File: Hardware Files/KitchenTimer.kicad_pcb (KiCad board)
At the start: 2 copper layers, 100 x 100 mm, 89 parts, among them J1 Conn_01x04, J2 USB_B_Micro, J3 Battery, Q1 P 1V 250uA 4A SOT-23, Q10 Q_NMOS_GSD, Q11 Q_NMOS_GSD, Q12 Q_NMOS_GSD, Q13 Q_NMOS_GSD, Q14 -30V 12A 14mΩ @ 8A, Q15 20V 7.5A 24mΩ @ 2.5Vgs, Q2 P 1V 250uA 4A SOT-23, Q3 P 1V 250uA 4A SOT-23, Q4 P 1V 250uA 4A SOT-23, Q5 P 1V 250uA 4A SOT-23, Q6 Q_NMOS_GSD, Q7 Q_NMOS_GSD, Q8 Q_NMOS_GSD, Q9 Q_NMOS_GSD, SW1 SW_SPST, SW2 SW_SPST, SW3 SW_Push_Dual, SW4 SW_Push_Dual, SW5 SW_Push_Dual, SW6 SW_Push_Dual, U1 74HC595, U2 74HC595, U3 ESP-WROOM-02D, U4 AP34063S8G-13, U5 TP4056, U6 AP9101CK6, U7 NCP1117ST50T3G, U8 NCP1117ST33T3G

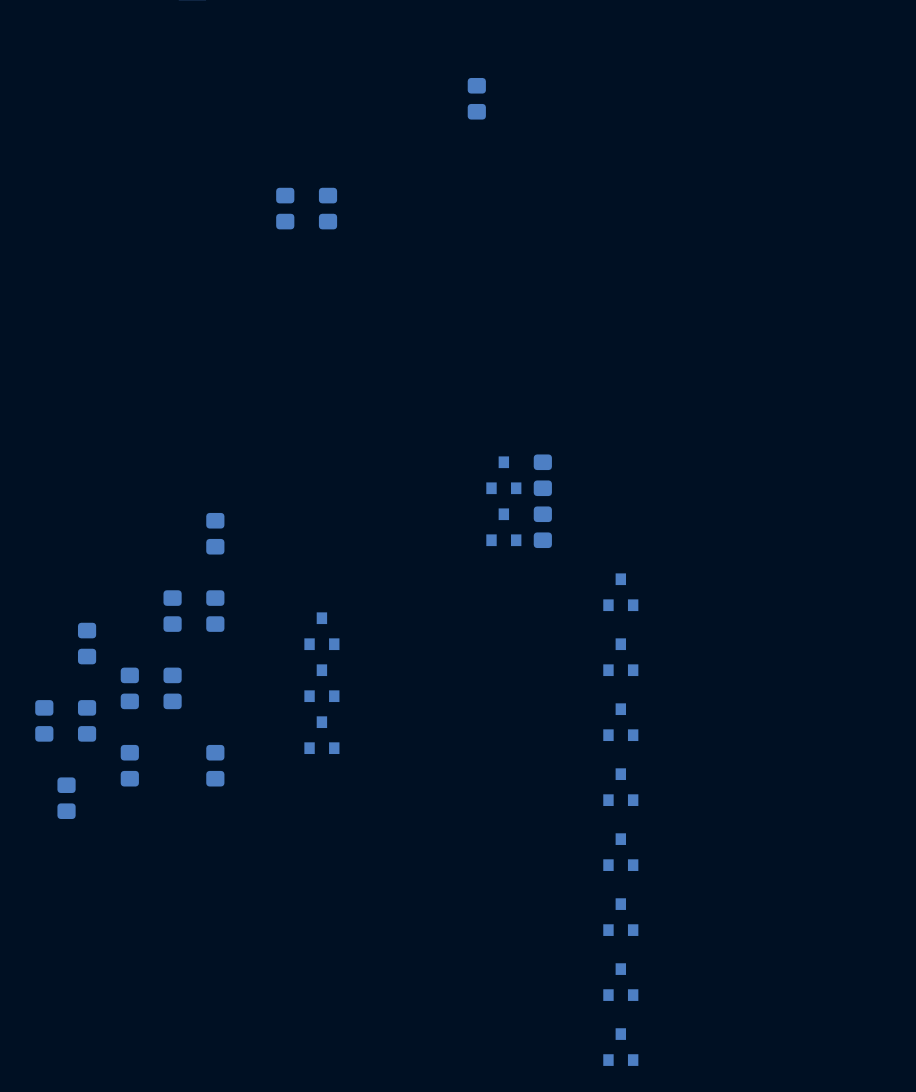
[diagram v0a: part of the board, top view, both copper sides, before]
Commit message: fix ground naming
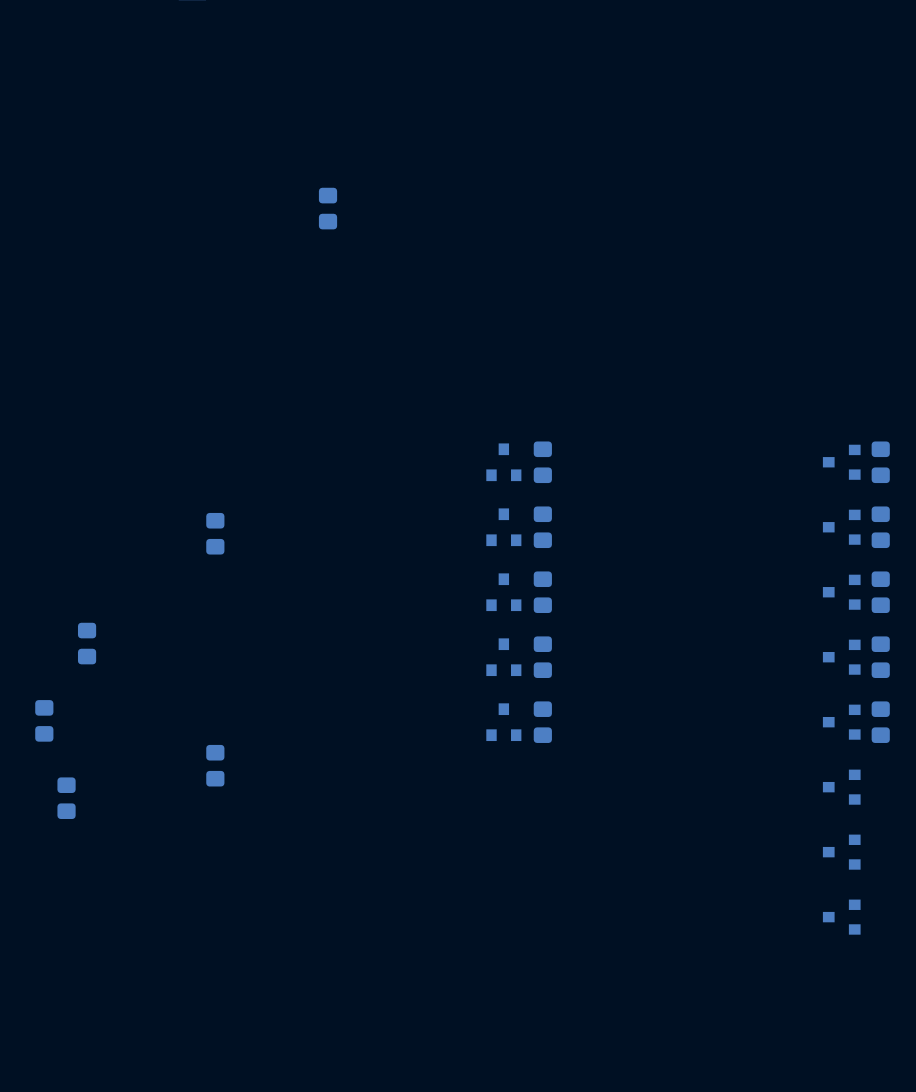
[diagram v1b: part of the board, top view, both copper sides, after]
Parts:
- moved R24 62.9 mm to (218.0, 67.0), turned to 270 degrees
- moved R25 58.3 mm to (218.0, 72.0), turned to 270 degrees
- moved R26 57.4 mm to (218.0, 77.0), turned to 270 degrees
- moved R27 55.2 mm to (218.0, 82.0), turned to 270 degrees
- moved R23 52.5 mm to (218.0, 62.0), turned to 270 degrees
- moved R20 38.3 mm to (192.0, 72.0)
- moved R22 32.0 mm to (192.0, 82.0)
- moved R21 28.6 mm to (192.0, 77.0)
- moved Q10 19.7 mm to (215.0, 82.0), turned to 180 degrees
- moved Q11 19.7 mm to (215.0, 87.0), turned to 180 degrees
- moved Q12 19.7 mm to (215.0, 92.0), turned to 180 degrees
- moved Q13 19.7 mm to (215.0, 97.0), turned to 180 degrees
- moved Q6 19.7 mm to (215.0, 62.0), turned to 180 degrees
- moved Q7 19.7 mm to (215.0, 67.0), turned to 180 degrees
- moved Q8 19.7 mm to (215.0, 72.0), turned to 180 degrees
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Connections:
- net LED_':'_Sink renamed GND

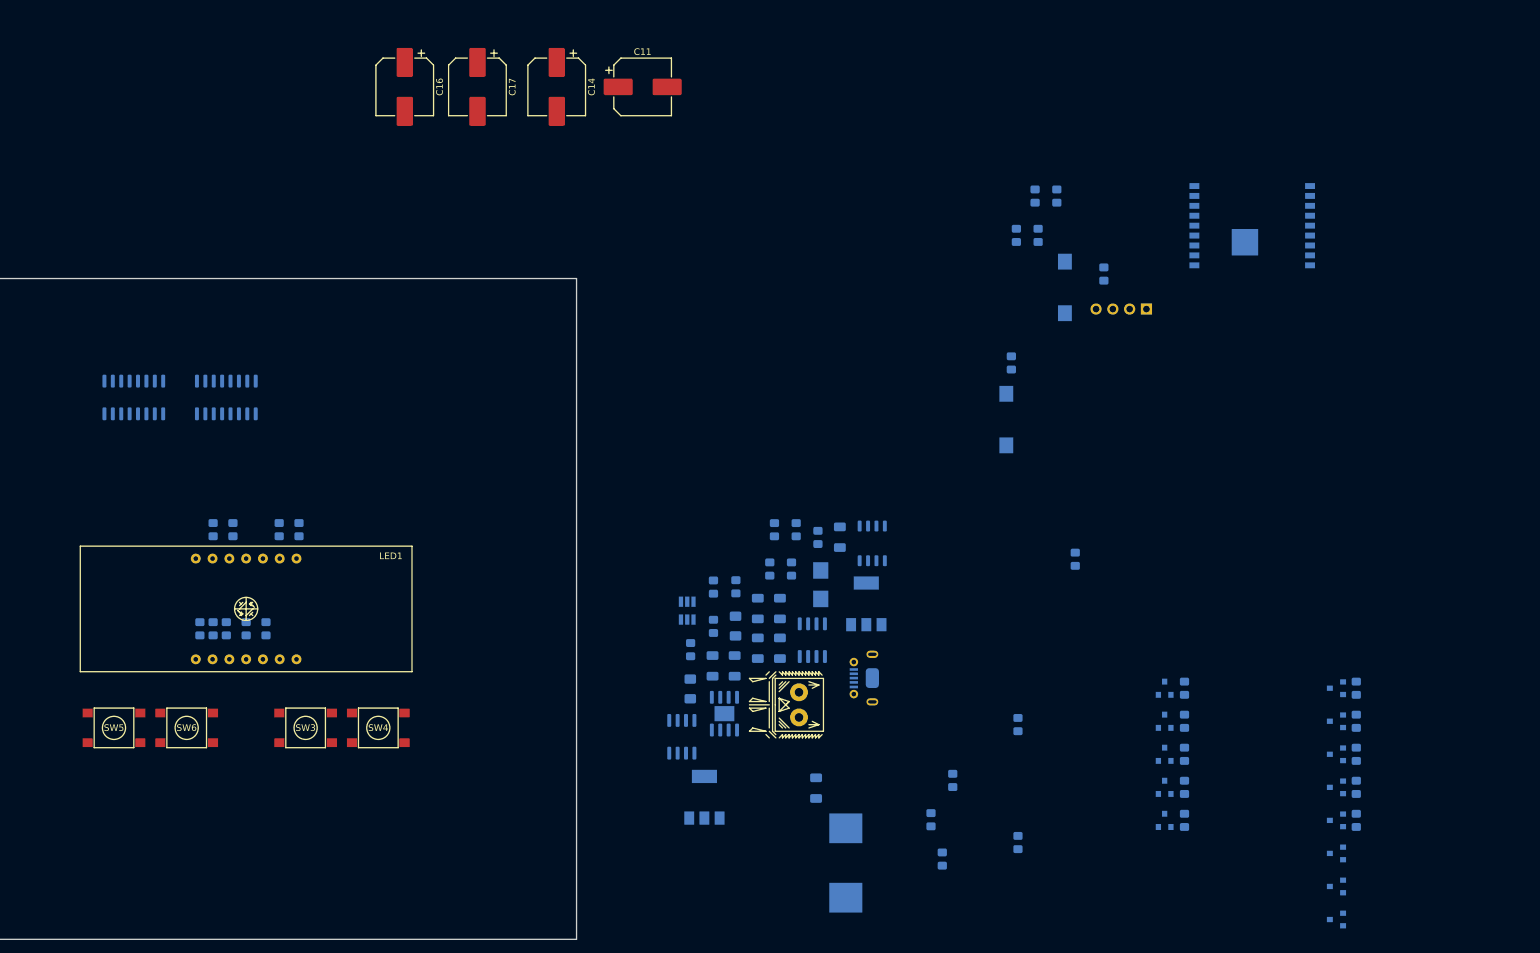
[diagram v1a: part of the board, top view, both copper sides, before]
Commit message: update layout
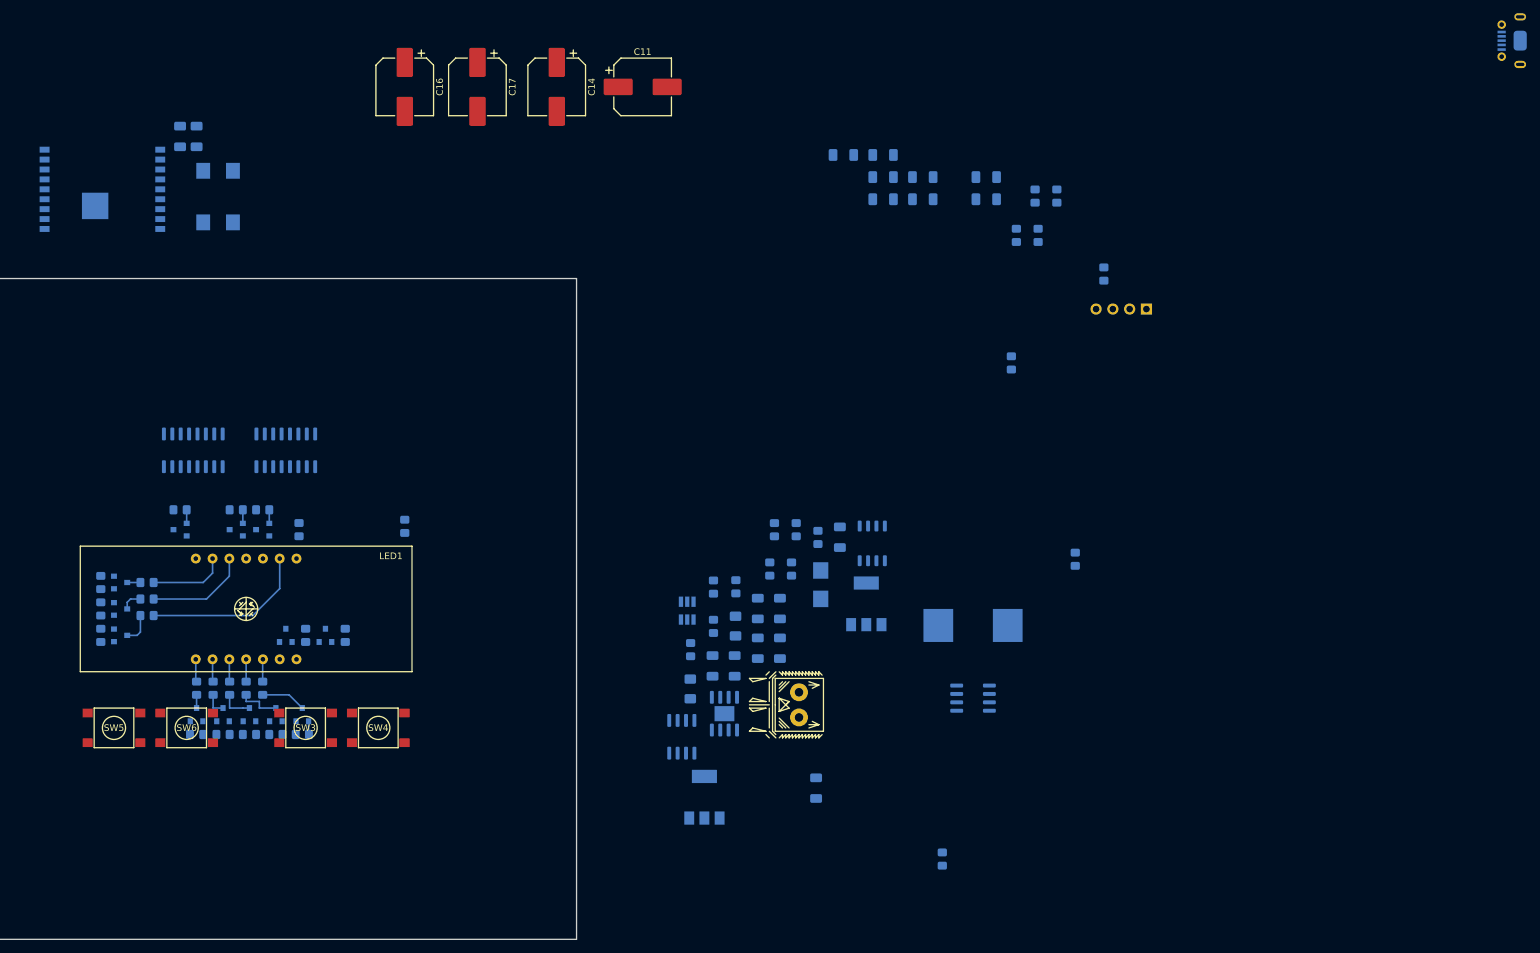
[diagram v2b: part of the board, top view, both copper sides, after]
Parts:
- added C1: 1uF, Capacitor_SMD:C_1206_3216Metric_Pad1.33x1.80mm_HandSolder, B.Cu at (162.0, -12.0)
- added C10: 1uF, Capacitor_SMD:C_1206_3216Metric_Pad1.33x1.80mm_HandSolder, B.Cu at (152.4, -15.3)
- added C2: 1uF, Capacitor_SMD:C_1206_3216Metric_Pad1.33x1.80mm_HandSolder, B.Cu at (162.0, -15.3)
- added C3: 1uF, Capacitor_SMD:C_1206_3216Metric_Pad1.33x1.80mm_HandSolder, B.Cu at (40.0, -21.5)
- added C4: 10uF, Capacitor_SMD:C_1206_3216Metric_Pad1.33x1.80mm_HandSolder, B.Cu at (42.5, -21.5)
- added C5: 1uF, Capacitor_SMD:C_1206_3216Metric_Pad1.33x1.80mm_HandSolder, B.Cu at (146.4, -12.0)
- added C6: 1uF, Capacitor_SMD:C_1206_3216Metric_Pad1.33x1.80mm_HandSolder, B.Cu at (140.4, -18.7)
- added C7: 1uF, Capacitor_SMD:C_1206_3216Metric_Pad1.33x1.80mm_HandSolder, B.Cu at (146.4, -15.3)
- added C8: 1uF, Capacitor_SMD:C_1206_3216Metric_Pad1.33x1.80mm_HandSolder, B.Cu at (152.4, -12.0)
- added C9: 1uF, Capacitor_SMD:C_1206_3216Metric_Pad1.33x1.80mm_HandSolder, B.Cu at (146.4, -18.7)
- moved R23 190.7 mm to (28.0, 46.0), turned to 90 degrees
- moved R24 190.4 mm to (28.0, 54.0), turned to 90 degrees
- moved Q11 187.7 mm to (31.0, 50.0), turned to 0 degrees
- moved Q6 184.7 mm to (31.0, 46.0), turned to 0 degrees
- moved Q7 184.5 mm to (31.0, 54.0), turned to 0 degrees
- moved R27 176.0 mm to (42.5, 69.0), turned to 180 degrees
- moved U3 174.1 mm to (37.0, -19.5)
- moved Q10 173.2 mm to (42.5, 66.0), turned to 90 degrees
- moved R26 171.7 mm to (46.5, 69.0), turned to 180 degrees
- moved Q9 168.9 mm to (46.5, 66.0), turned to 90 degrees
- moved Q13 167.4 mm to (50.5, 66.0), turned to 90 degrees
- moved R25 163.5 mm to (54.5, 69.0), turned to 180 degrees
- moved Q8 160.6 mm to (54.5, 66.0), turned to 90 degrees
- moved Q12 158.6 mm to (58.5, 66.0), turned to 90 degrees
- moved R18 154.4 mm to (40.0, 35.0), turned to 180 degrees
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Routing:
- net Net-(LED1-Pad9): track 0.00 -> 25.3 mm
- net Net-(LED1-Pad12): track 0.00 -> 15.6 mm
- net Net-(LED1-Pad13): track 0.00 -> 11.7 mm
- net LED_G_Sink: track 0.00 -> 6.83 mm
- net LED_C_Sink: track 0.00 -> 6.50 mm
- net LED_DP_Sink: track 0.00 -> 5.00 mm
- net LED_B_Sink: track 0.00 -> 4.71 mm
- net LED_D_Sink: track 0.00 -> 3.50 mm
- net Net-(LED1-Pad1): track 0.00 -> 3.43 mm
- net Net-(LED1-Pad2): track 0.00 -> 3.41 mm
- net Net-(LED1-Pad5): track 0.00 -> 3.40 mm
- net Net-(LED1-Pad3): track 0.00 -> 3.40 mm
- net Net-(LED1-Pad4): track 0.00 -> 3.38 mm
- net LED_F_Sink: track 0.00 -> 3.21 mm
- net Char_3: track 0.00 -> 2.05 mm
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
